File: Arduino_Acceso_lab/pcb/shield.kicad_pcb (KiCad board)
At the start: 2 copper layers, 83.6 x 59.4 mm, 29 parts, among them K1 RELAY_C, K2 RELAY_C, P1 Power, P13 Timer RTC, P14 Sensor1, P15 Sensor2, P16 Luz1, P17 Luz2, P2 Analog, P3 Digital, P4 Digital, Q1 2N2222, Q2 2N2222

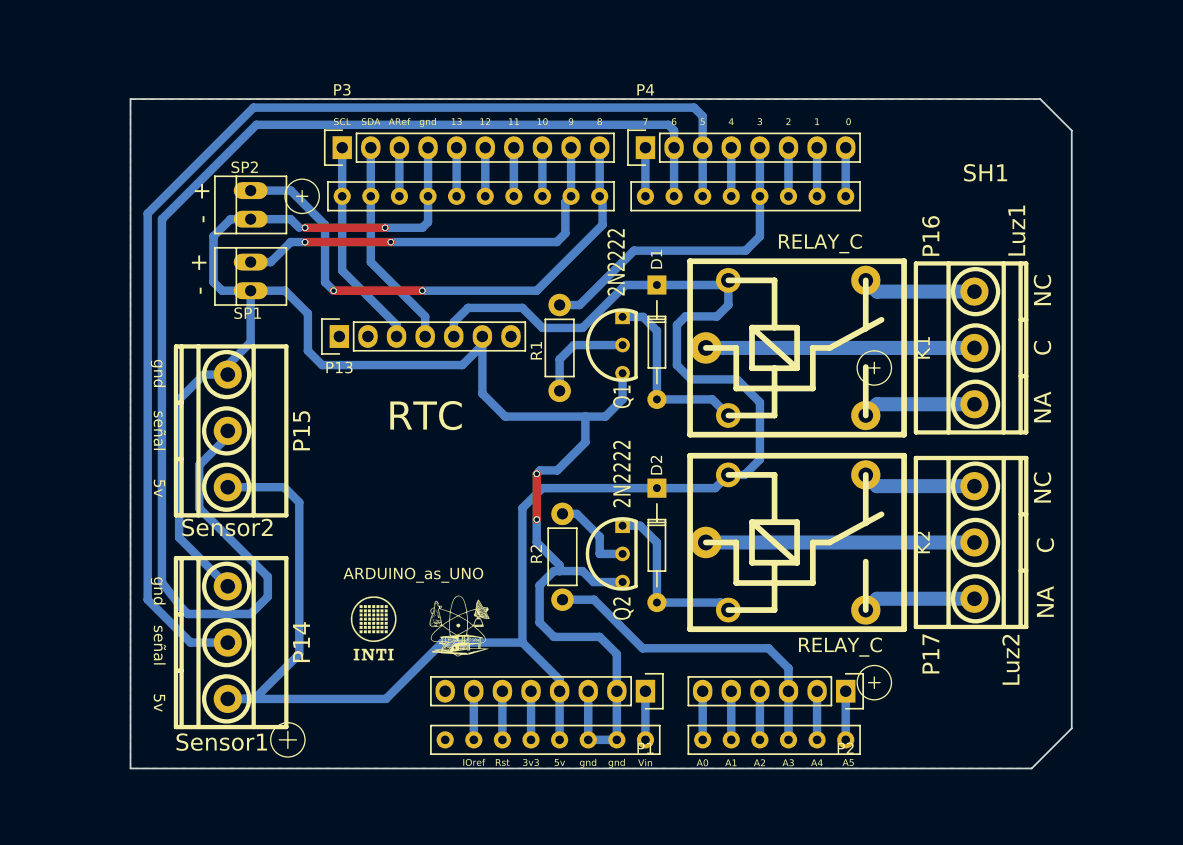
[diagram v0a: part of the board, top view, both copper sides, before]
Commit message: Arduino Acceso Lab. Ultimas modificaciones al PCB.
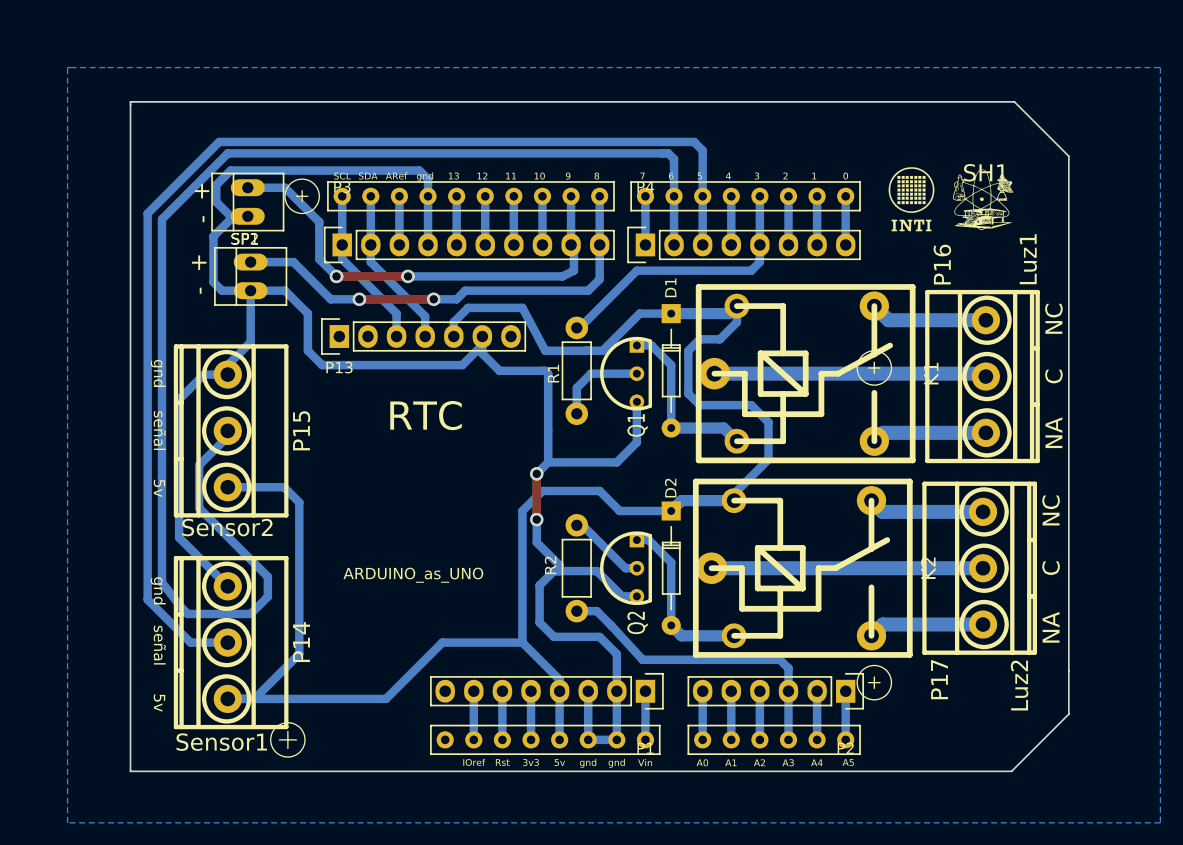
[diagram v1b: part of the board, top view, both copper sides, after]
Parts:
- removed the G*** at (114.0, 70.0)
- removed the G*** at (184.4, 74.3)
- moved G*** 61.1 mm to (180.6, 75.6)
- moved G*** 59.9 mm to (186.9, 75.6)
- moved P3 8.64 mm to (130.0, 79.6)
- moved P4 8.64 mm to (157.0, 79.6)
- moved SP1 6.61 mm to (121.7, 75.8)
- moved SP2 6.35 mm to (121.9, 82.4)
- moved D1 2.84 mm to (159.3, 85.7)
- moved Q1 2.84 mm to (156.2, 91.1)
- moved P16 2.74 mm to (187.2, 91.3)
- moved R1 2.54 mm to (150.9, 94.6)
- moved K1 2.41 mm to (171.2, 91.1)
- moved P17 2.41 mm to (186.9, 108.3)
- moved D2 2.40 mm to (159.3, 103.3)
- moved K2 2.34 mm to (170.9, 108.3)
- moved Q2 1.80 mm to (156.2, 108.3)
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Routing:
- net /gnd: track 165.9 -> 176.9 mm, vias 4 -> 2
- net Net-(P3-Pad10): track 47.3 -> 40.8 mm
- net Net-(P13-Pad4): track 18.8 -> 14.4 mm
- net Net-(P13-Pad3): track 18.8 -> 14.4 mm
- net Net-(P3-Pad9): track 37.2 -> 41.3 mm
- net /3(**): track 28.2 -> 25.6 mm
- net /5v: track 155.5 -> 157.6 mm
- net /A3: track 28.9 -> 27.3 mm
- net Net-(D1-Pad2): track 16.6 -> 15.7 mm
- net Net-(Q2-Pad2): track 7.70 -> 6.91 mm
- net Net-(Q1-Pad2): track 8.91 -> 8.15 mm
- net Net-(P15-Pad2): track 116.9 -> 117.6 mm
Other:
- board size 83.6 x 59.4 mm -> 83.3 x 59.4 mm

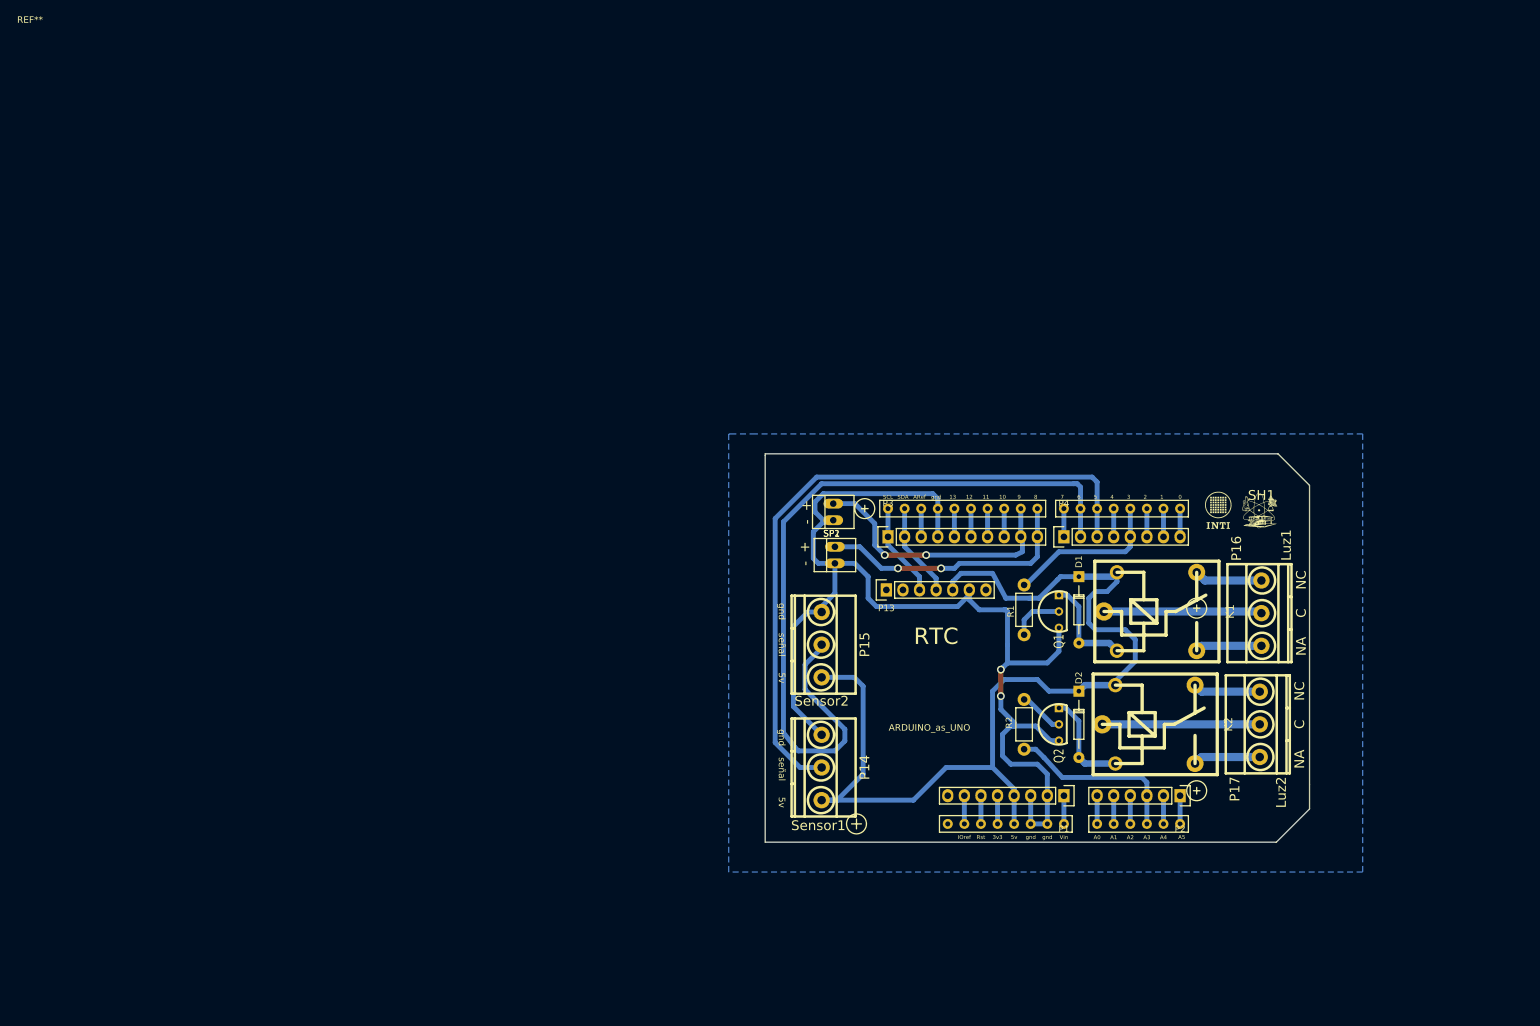
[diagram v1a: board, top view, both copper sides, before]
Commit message: Nuevo PCB.
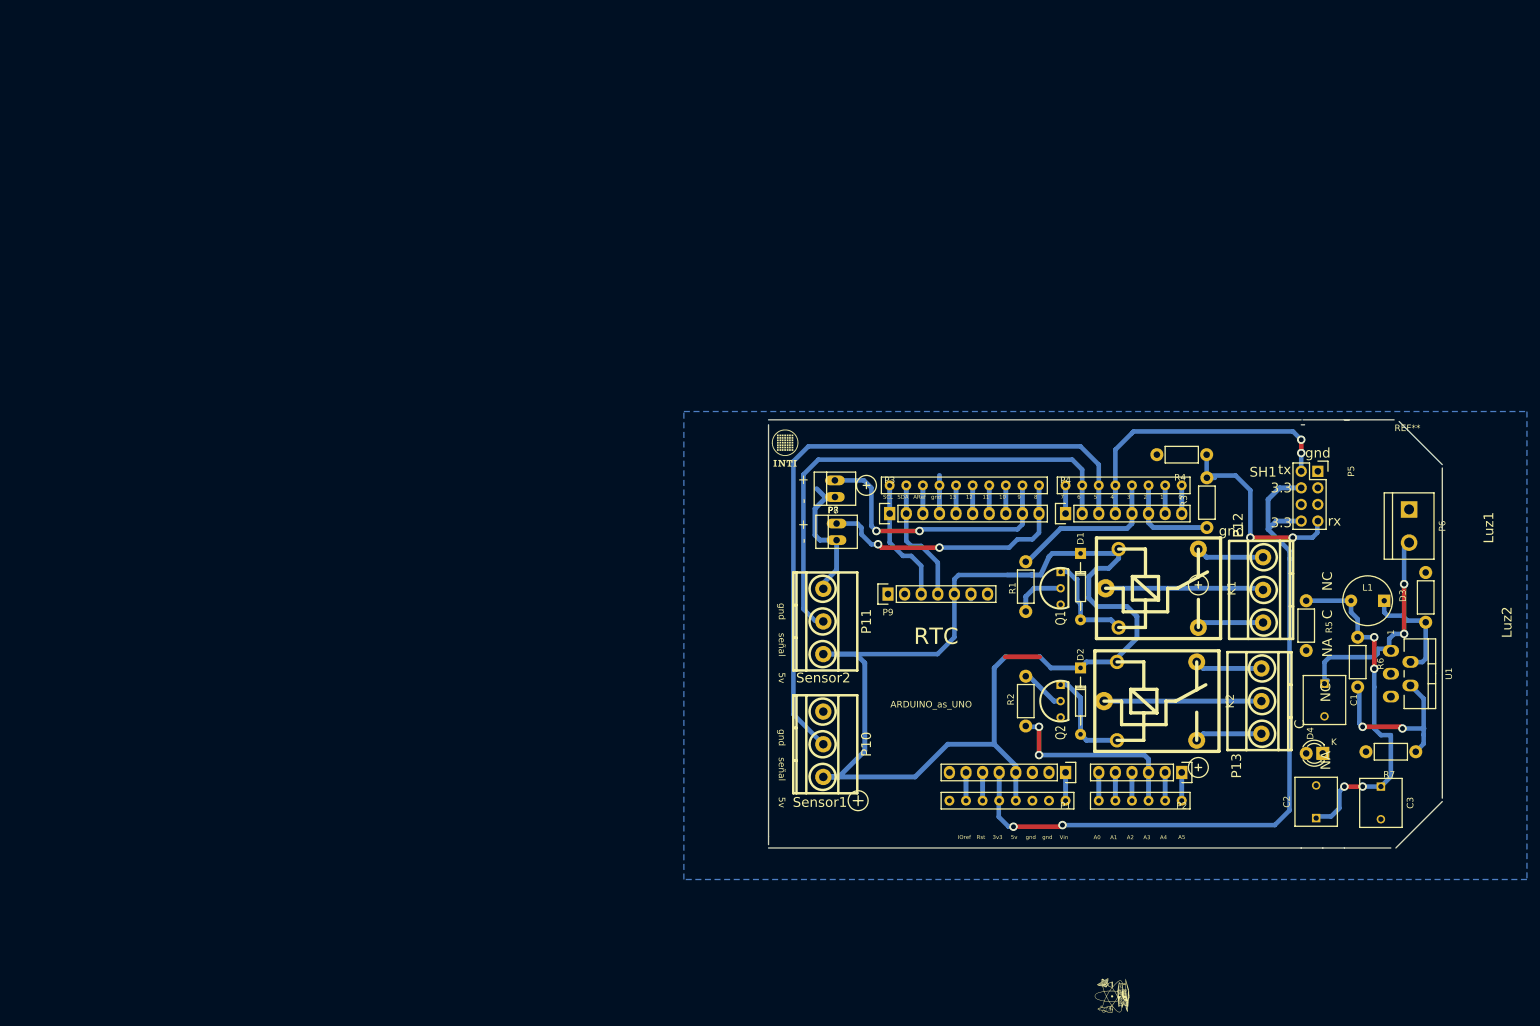
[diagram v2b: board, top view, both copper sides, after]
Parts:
- added C1: CP1, Capacitors_ThroughHole:C_Rect_L7.5_W6.5_P5, F.Cu at (196.8, 102.1)
- added C2: CP1, Capacitors_ThroughHole:C_Rect_L7.5_W6.5_P5, F.Cu at (195.6, 122.7)
- added C3: C, Capacitors_ThroughHole:C_Rect_L7.5_W6.5_P5, F.Cu at (205.5, 117.9)
- added D3: D, Resistors_ThroughHole:Resistor_Horizontal_RM7mm, F.Cu at (212.3, 92.7)
- added D4: LED, LEDs:LED-3MM, F.Cu at (196.6, 112.8)
- added L1: INDUCTOR, Inductors:INDUCTOR_V, F.Cu at (203.5, 89.4)
- added P5: modulo esp8266, Socket_Strips:Socket_Strip_Straight_2x04, F.Cu at (195.8, 69.6)
- added P6: fuente, Connect:bornier2, F.Cu at (209.8, 78.0)
- added R3: R, Resistors_ThroughHole:Resistor_Horizontal_RM7mm, F.Cu at (178.9, 78.2)
- added R4: R, Resistors_ThroughHole:Resistor_Horizontal_RM7mm, F.Cu at (178.8, 67.1)
- added R5: R, Resistors_ThroughHole:Resistor_Horizontal_RM7mm, F.Cu at (194.1, 89.4)
- added R6: R, Resistors_ThroughHole:Resistor_Horizontal_RM7mm, F.Cu at (201.9, 95.0)
- added R7: R, Resistors_ThroughHole:Resistor_Horizontal_RM7mm, F.Cu at (210.8, 112.5)
- added U1: LM2576, TO_SOT_Packages_THT:Pentawatt_Neutral_Staggered_Verical_TO220-5-T05D, F.Cu at (210.8, 100.6)
- P7: renamed from SP1; value buzzer2 -> buzzer 1
- P8: renamed from SP2; value buzzer1 -> buzzer 2
- moved ? 219.9 mm to (210.8, 62.5) (x4)
- moved REF** 219.9 mm to (210.8, 62.5)
- moved G*** 77.7 mm to (164.3, 149.9), turned to 90 degrees
- moved G*** 67.0 mm to (114.3, 66.0)
- moved D2 3.57 mm to (159.5, 99.7)
- moved P3 3.57 mm to (130.3, 76.1)
- moved P4 3.57 mm to (157.2, 76.1)
- moved P13 3.57 mm to (187.2, 104.8)
- moved P7 3.57 mm to (121.9, 72.3)
- moved P8 3.57 mm to (122.2, 78.9)
- moved D1 3.57 mm to (159.5, 82.2)
- moved K1 3.57 mm to (171.4, 87.5)
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- renumbered P14 to P10, P15 to P11, P16 to P12, P17 to P13, P13 to P9
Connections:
- net /5v renamed +5P
- net Net-(P1-Pad5) renamed +3.3VP
- net Net-(P4-Pad4) renamed /rx-wifi
- net Net-(P4-Pad6) renamed /tx-wifi
- P1 pad 2: /gnd -> GNDD
- P1 pad 3: /gnd -> GNDD
- P10 pad 1: /gnd -> GNDD
- P11 pad 1: /gnd -> GNDD
- P3 pad 4: /gnd -> Net-(P3-Pad4)
- P7 pad 1: /gnd -> GNDD
- P8 pad 1: /gnd -> GNDD
- P9 pad 6: /gnd -> GNDD
- Q1 pad 1: /gnd -> GNDD
- Q2 pad 1: /gnd -> GNDD
- SH1 pad GND1: /gnd -> GNDD
- SH1 pad GND2: /gnd -> GNDD
- SH1 pad GND3: /gnd -> Net-(P3-Pad4)
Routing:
- net /gnd: track 176.9 -> 0.00 mm, vias 2 -> 0
- net +3.3VP: track 4.32 -> 113.4 mm, vias 0 -> 2
- net Net-(C2-Pad1): track 0.00 -> 54.6 mm, vias 0 -> 4
- net Net-(P11-Pad2): track 117.6 -> 75.9 mm
- net /rx-wifi: track 4.32 -> 44.8 mm, vias 0 -> 2
- net Net-(C1-Pad1): track 0.00 -> 35.5 mm, vias 0 -> 2
- net Net-(P5-Pad7): track 0.00 -> 32.1 mm, vias 0 -> 2
- net Net-(R6-Pad2): track 0.00 -> 27.4 mm, vias 0 -> 2
- net GNDD: track 0.00 -> 24.4 mm, vias 0 -> 1
- net +5P: track 157.6 -> 179.8 mm
- net Net-(D3-Pad1): track 0.00 -> 16.9 mm
- net /tx-wifi: track 4.32 -> 15.0 mm
- net Net-(P3-Pad4): track 0.00 -> 5.84 mm
- net (no net): track 0.00 -> 5.25 mm
- net Net-(P3-Pad2): track 14.4 -> 19.5 mm
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- added copper zone on B.Cu, net GNDD
- removed copper zone on B.Cu, net /gnd
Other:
- board size 83.3 x 59.4 mm -> 103.1 x 65.5 mm
- net class Default: clearance 0.2 -> 0.7; trace_width 0.25 -> 0.7; via_dia 0.6 -> 1.3; via_drill 0.4 -> 0.75
- rule trace_clearance: 0.2 -> 0.7
- rule trace_min: 0.2 -> 0.7
- rule via_min_drill: 0.3 -> 0.75
- rule via_min_size: 0.4 -> 1.3
- board text added: "3.3"
- board text added: "rx"
- board text added: "tx"
